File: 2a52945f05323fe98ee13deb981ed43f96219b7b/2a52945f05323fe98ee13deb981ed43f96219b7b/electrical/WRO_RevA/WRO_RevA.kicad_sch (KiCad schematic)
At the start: 22 parts, among them J1 VCC, J2 MPU6050, J3 TO_PI, J4 SERVO, J5 MOTOR, SW1 EXEC_PRGM, U1 ESP32-DEVKITC-32D, U2 ROB-14450, U3 BOB-12009

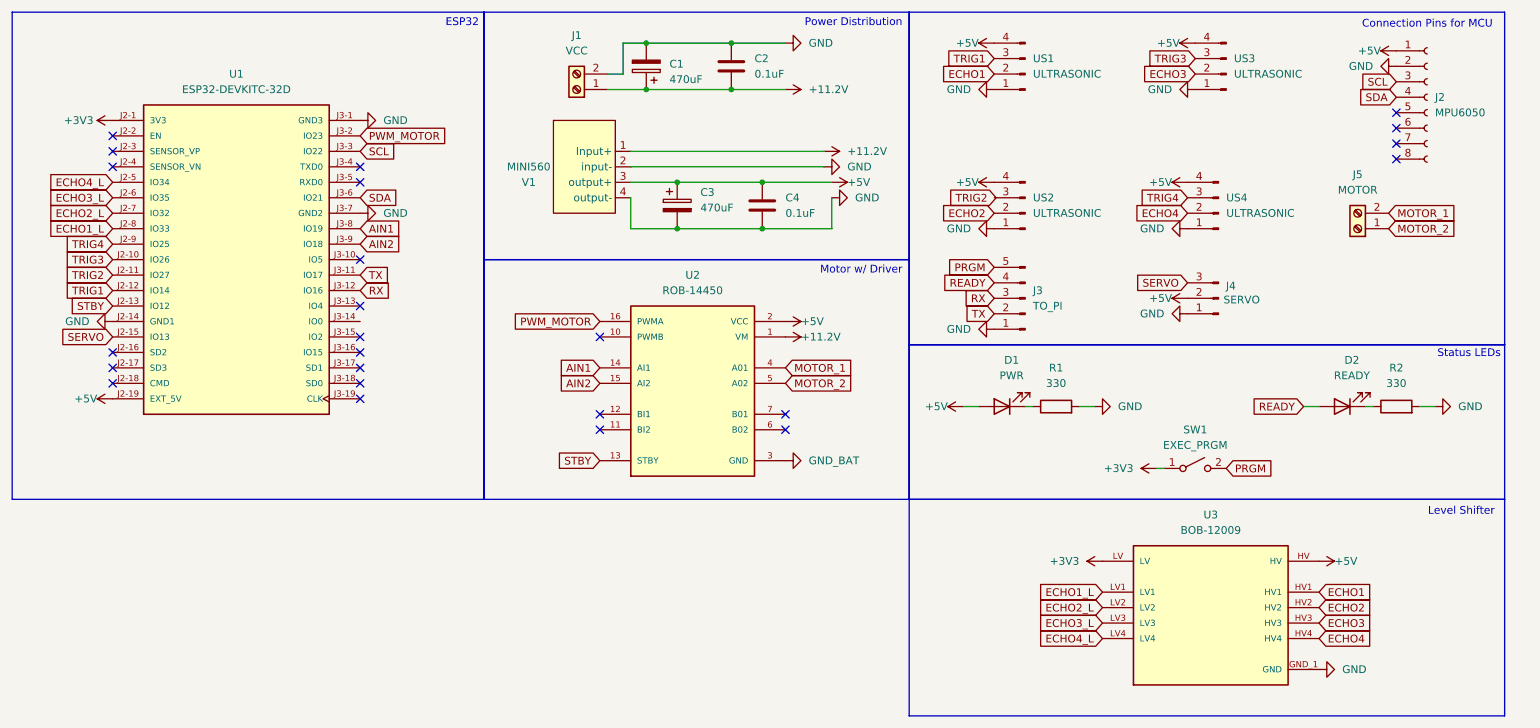
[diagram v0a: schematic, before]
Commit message: final shape for PCB, only need to route
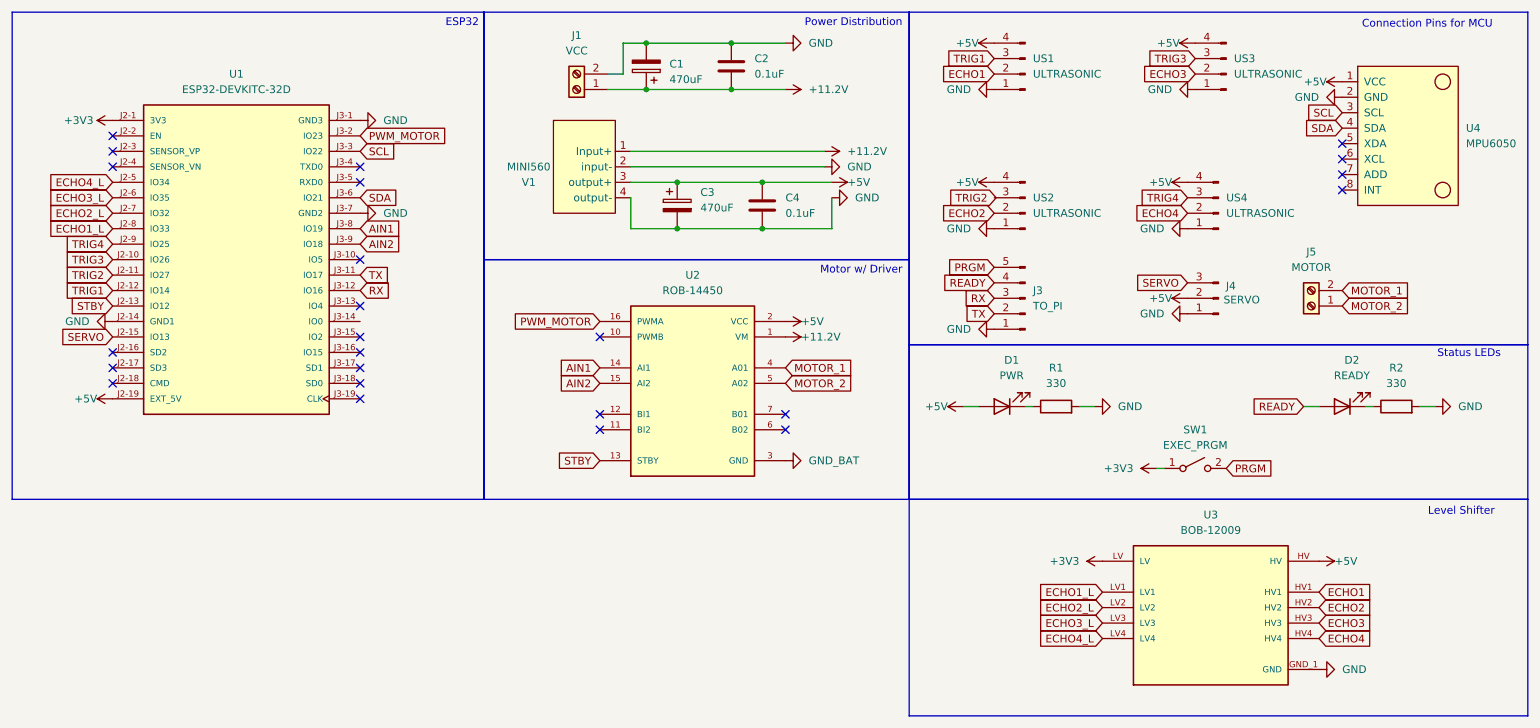
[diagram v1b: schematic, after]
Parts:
- removed J2: MPU6050, Connector_PinSocket_2.54mm:PinSocket_1x08_P2.54mm_Vertical, symbol Connector:Conn_01x08_Socket
- added U4: MPU6050, usini_sensors:module_mpu6050, symbol usini_sensors:module_mpu6050
- US1, US2, US3, US4: footprint Connector_PinSocket_2.54mm:PinSocket_1x04_P2.54mm_Vertical -> Connector_PinHeader_2.54mm:PinHeader_1x04_P2.54mm_Vertical
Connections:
- net +5V: now also U4.1 (VCC)
- net GND: now also U4.2 (GND)
- net SCL: now also U4.3 (SCL)
- net SDA: now also U4.4 (SDA)
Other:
- moved on the sheet: J5
